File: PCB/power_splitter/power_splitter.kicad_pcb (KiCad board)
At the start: 2 copper layers, 56 x 48 mm, 34 parts, among them J1 B02P-VL, J2 B02P-VL, J3 B02P-VL, J4 PJ-082BH, J5 B02P-VL, Q2 IRLZ44N, U1 AP62300TWU, U2 AP62300TWU

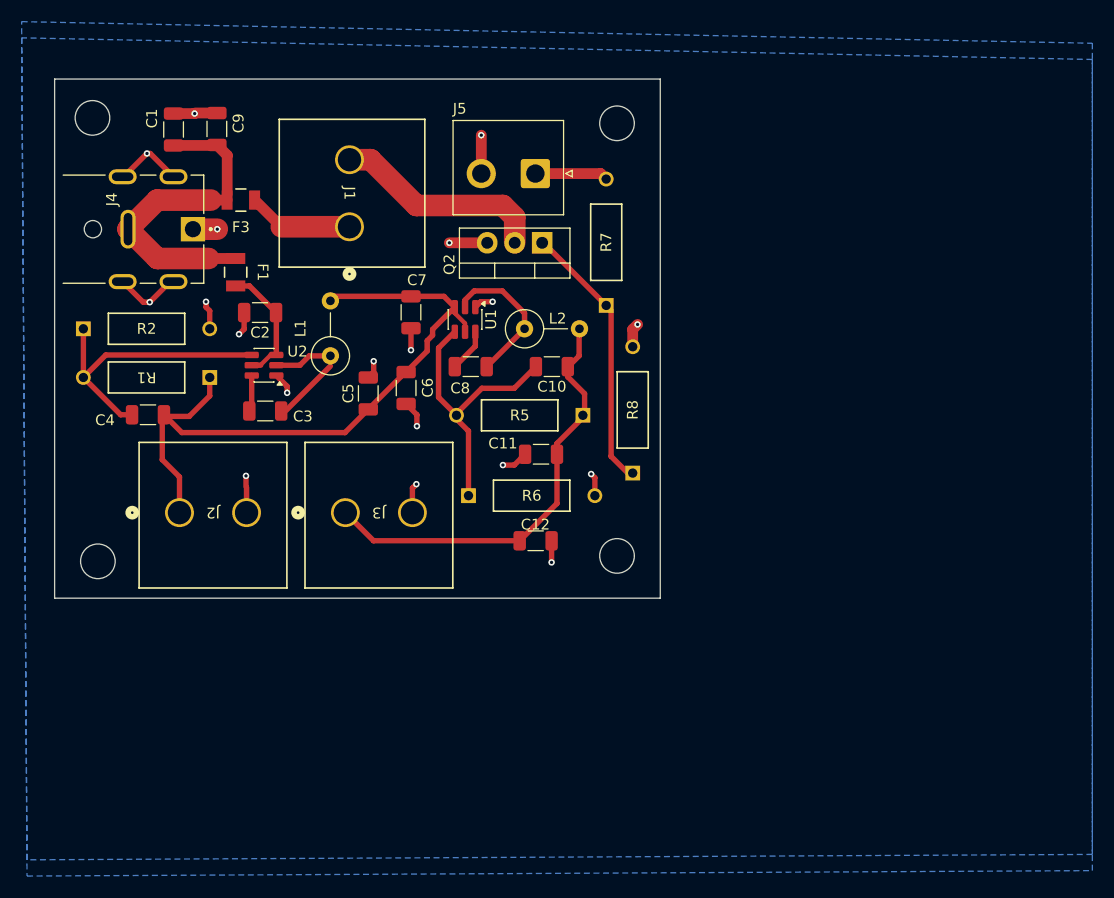
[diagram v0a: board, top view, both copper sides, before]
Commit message: Liv's stuff
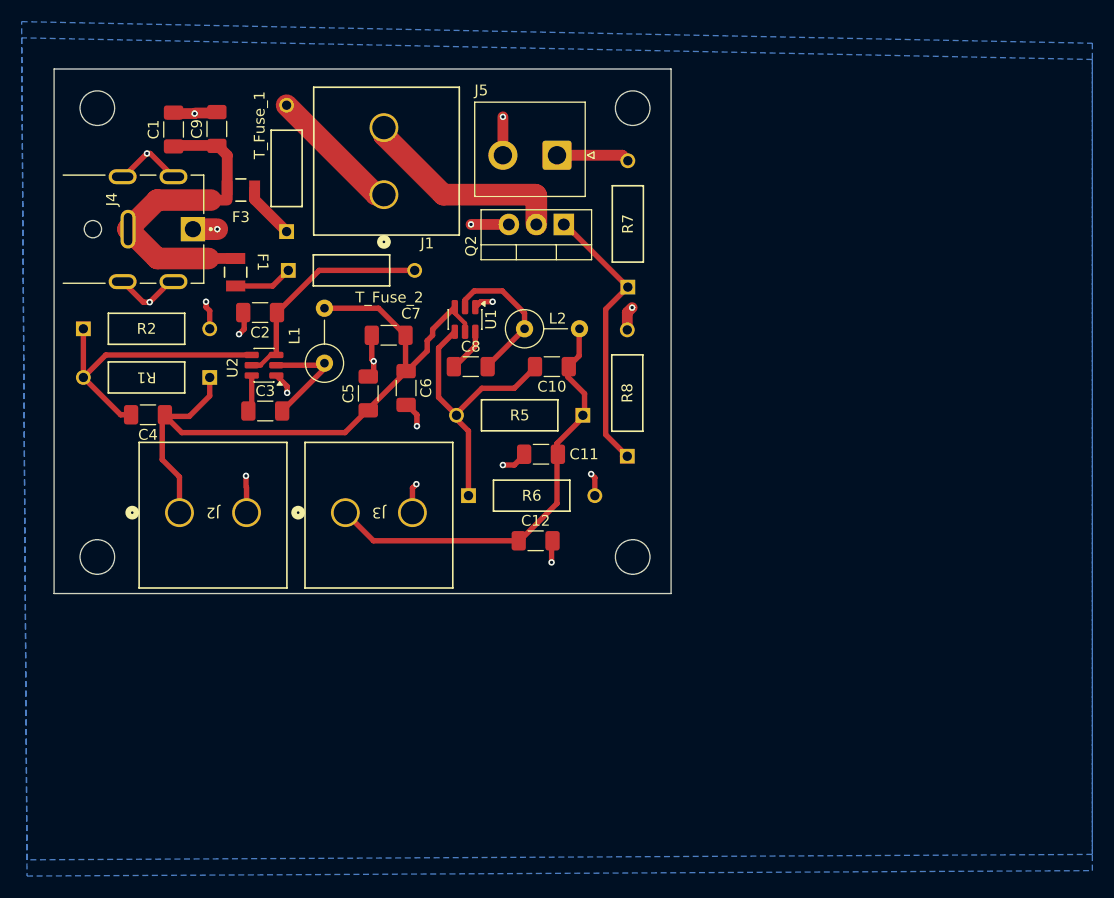
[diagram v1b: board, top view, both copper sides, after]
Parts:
- added T_Fuse_1: R_Small, RESISTOR:YAG_MF25_YAG, F.Cu at (99.0, 44.4)
- added T_Fuse_2: R_Small, RESISTOR:YAG_MF25_YAG, F.Cu at (99.2, 48.0)
- C1, C10, C11, C12, C2, C3, C4, C5, C6, C7, C8, C9: footprint Capacitor_SMD:C_1206_3216Metric -> Capacitor_SMD:C_1206_3216Metric_Pad1.33x1.80mm_HandSolder
- moved J1 4.35 mm to (108.0, 41.0)
- moved C7 2.96 mm to (108.4, 54.0), turned to 180 degrees
- moved Q2 2.62 mm to (124.6, 43.8)
- moved J5 2.62 mm to (124.0, 37.4)
- moved R7 2.62 mm to (130.6, 49.5)
- moved REF** 2.02 mm to (131.0, 33.0)
- moved R8 1.64 mm to (130.5, 65.2)
- moved REF** 1.45 mm to (131.0, 74.5)
- moved REF** 1.01 mm to (81.5, 33.0)
- moved F3 0.93 mm to (94.8, 40.6)
- moved L1 0.87 mm to (102.5, 56.6)
- moved REF** 0.40 mm to (81.5, 74.5)
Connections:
- F1 pad 2: Net-(U2-EN) -> Net-(F1-Pad2)
- J1 pad 1: Net-(F3-Pad2) -> Net-(J1-Pad1)
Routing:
- net Net-(J1-Pad1): track 0.00 -> 12.4 mm
- net Net-(U2-EN): track 11.4 -> 21.0 mm
- net Net-(F1-Pad2): track 0.00 -> 5.46 mm
- net Net-(F3-Pad2): track 9.80 -> 5.07 mm
- net Net-(U2-SW): track 11.9 -> 10.6 mm
- net Net-(Q2-G): track 25.1 -> 26.1 mm
- net GND: track 55.7 -> 56.1 mm, vias 19 -> 18
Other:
- board size 56 x 48 mm -> 57.1 x 48.5 mm
